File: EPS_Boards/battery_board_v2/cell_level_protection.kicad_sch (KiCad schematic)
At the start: 32 parts, among them J8 Shunt Resistor, Q10 CSD16406Q3, Q3 CSD16406Q3, Q4 CSD16406Q3, Q5 CSD16406Q3, Q6 CSD16406Q3, Q7 CSD16406Q3, Q8 CSD16406Q3, Q9 CSD16406Q3, U10 BQ29723, U11 BQ29723, U8 BQ29723, U9 BQ29723

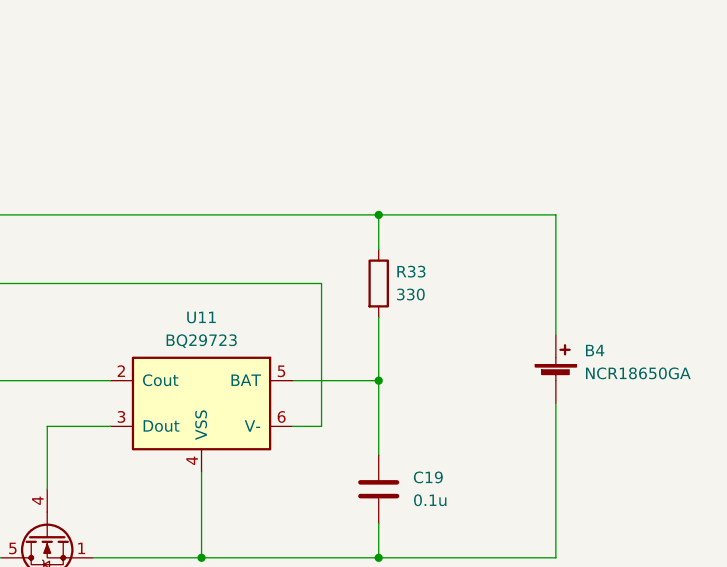
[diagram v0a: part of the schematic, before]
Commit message: eps:battery:pcb layout
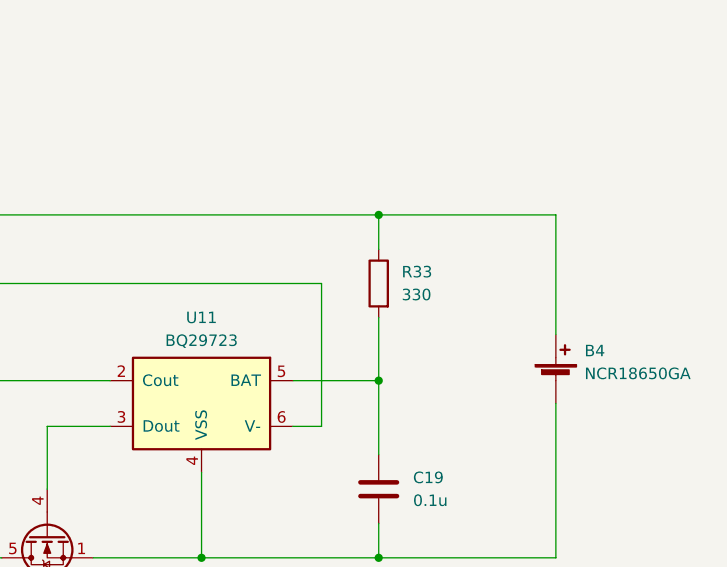
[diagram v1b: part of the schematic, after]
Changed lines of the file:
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@@
     (pin "2")
   )
-  (symbol (lib_id "Device:R") (at 299.72 114.3 0) (unit 1)
+  (symbol (lib_id "Device:R") (at 299.72 114.3 0) (mirror y) (unit 1)
     (in_bom yes) (on_board yes) (fields_autoplaced)
-    (property "Reference" "R33" (id 0) (at 301.625 113.0299 0)
-      (effects (font (size 1.27 1.27)) (justify left))
+    (property "Reference" "R33" (id 0) (at 302.26 113.0299 0)
+      (effects (font (size 1.27 1.27)) (justify right))
     )
-    (property "Value" "330" (id 1) (at 301.625 115.5699 0)
-      (effects (font (size 1.27 1.27)) (justify left))
+    (property "Value" "330" (id 1) (at 302.26 115.5699 0)
+      (effects (font (size 1.27 1.27)) (justify right))
     )
-    (property "Footprint" "Resistor_SMD:R_0402_1005Metric" (id 2) (at 297.942 114.3 90)
+    (property "Footprint" "Resistor_SMD:R_0402_1005Metric" (id 2) (at 301.498 114.3 90)
       (effects (font (size 1.27 1.27)) hide)
     )
